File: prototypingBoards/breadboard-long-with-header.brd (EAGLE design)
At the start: 99.1 x 56.5 mm, 85 parts

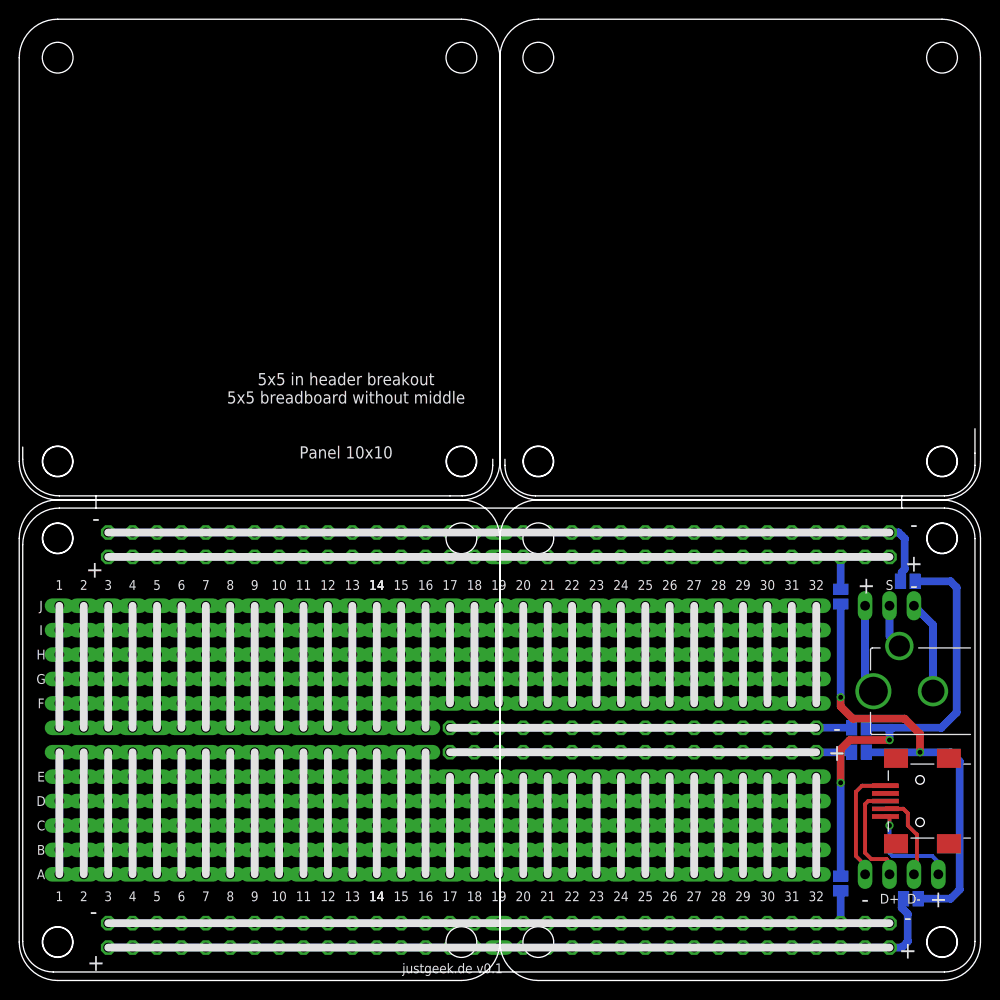
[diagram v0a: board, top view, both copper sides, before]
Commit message: Cleaned up boards
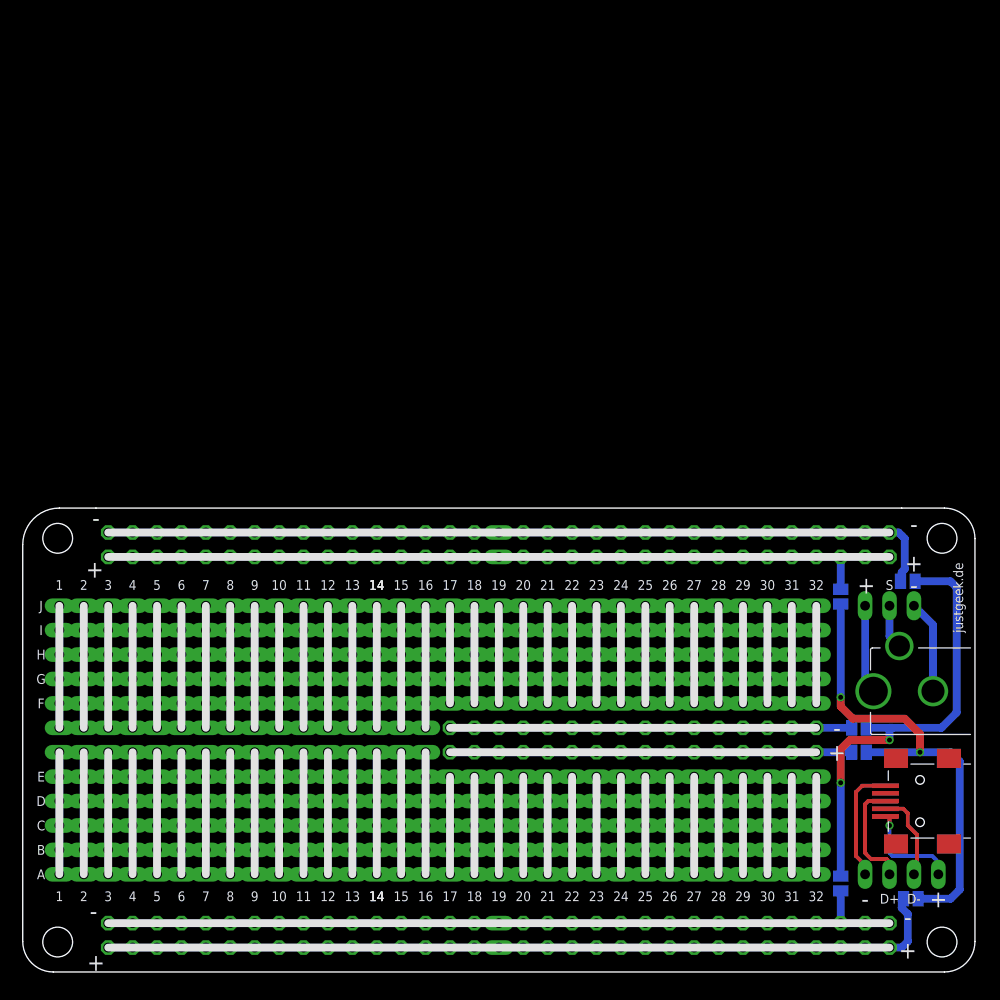
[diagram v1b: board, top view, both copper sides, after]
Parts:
- removed PCB1, PCB2, PCB3, PCB4: PCB_DP_SQUARE-5X5, dp_pcb:DP5050_V1
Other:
- board size 99.1 x 56.5 mm -> 99.1 x 48.3 mm
- board text added: "justgeek.de"
- board text removed: "5x5 in header breakout 5x5 breadboard without middle Panel 10x10"
- board text removed: "justgeek.de v0.1"
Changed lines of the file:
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@@
 <?xml version="1.0" encoding="utf-8"?>
 <!DOCTYPE eagle SYSTEM "eagle.dtd">
-<eagle version="6.5.0">
+<eagle version="7.1.0">
 <drawing>
 <settings>
@@
 <setting verticaltext="up"/>
 </settings>
-<grid distance="25" unitdist="mil" unit="mil" style="lines" multiple="1" display="yes" altdistance="5" altunitdist="mil" altunit="mil"/>
+<grid distance="1" unitdist="mm" unit="mm" style="lines" multiple="1" display="yes" altdistance="0.1" altunitdist="mm" altunit="mm"/>
 <layers>
 <layer number="1" name="Top" color="4" fill="1" visible="no" active="yes"/>
@@
 <layer number="19" name="Unrouted" color="6" fill="1" visible="no" active="yes"/>
 <layer number="20" name="Dimension" color="15" fill="1" visible="yes" active="yes"/>
-<layer number="21" name="tPlace" color="7" fill="1" visible="yes" active="yes"/>
+<layer number="21" name="tPlace" color="7" fill="1" visible="no" active="yes"/>
 <layer number="22" name="bPlace" color="7" fill="1" visible="yes" active="yes"/>
-<layer number="23" name="tOrigins" color="15" fill="1" visible="yes" active="yes"/>
+<layer number="23" name="tOrigins" color="15" fill="1" visible="no" active="yes"/>
 <layer number="24" name="bOrigins" color="15" fill="1" visible="no" active="yes"/>
-<layer number="25" name="tNames" color="7" fill="1" visible="yes" active="yes"/>
-<layer number="26" name="bNames" color="7" fill="1" visible="no" active="yes"/>
+<layer number="25" name="tNames" color="7" fill="1" visible="no" active="yes"/>
+<layer number="26" name="bNames" color="7" fill="1" visible="yes" active="yes"/>
 <layer number="27" name="tValues" color="7" fill="1" visible="no" active="yes"/>
-<layer number="28" name="bValues" color="7" fill="1" visible="no" active="yes"/>
-<layer number="29" name="tStop" color="7" fill="3" visible="yes" active="yes"/>
-<layer number="30" name="bStop" color="7" fill="6" visible="no" active="yes"/>
+<layer number="28" name="bValues" color="7" fill="1" visible="yes" active="yes"/>
+<layer number="29" name="tStop" color="7" fill="3" visible="no" active="yes"/>
+<layer number="30" name="bStop" color="7" fill="6" visible="yes" active="yes"/>
 <layer number="31" name="tCream" color="7" fill="4" visible="no" active="yes"/>
 <layer number="32" name="bCream" color="7" fill="5" visible="no" active="yes"/>
@@
 <layer number="43" name="vRestrict" color="2" fill="10" visible="no" active="yes"/>
 <layer number="44" name="Drills" color="7" fill="1" visible="no" active="yes"/>
-<layer number="45" name="Holes" color="7" fill="1" visible="yes" active="yes"/>
+<layer number="45" name="Holes" color="7" fill="1" visible="no" active="yes"/>
 <layer number="46" name="Milling" color="3" fill="1" visible="no" active="yes"/>
 <layer number="47" name="Measures" color="7" fill="1" visible="no" active="yes"/>
@@
 <layer number="109" name="ref-old" color="11" fill="1" visible="no" active="yes"/>
 <layer number="116" name="Patch_BOT" color="9" fill="4" visible="no" active="yes"/>
-<layer number="121" name="_tsilk" color="7" fill="1" visible="yes" active="yes"/>
-<layer number="122" name="_bsilk" color="7" fill="1" visible="no" active="yes"/>
+<layer number="121" name="_tsilk" color="7" fill="1" visible="no" active="yes"/>
+<layer number="122" name="_bsilk" color="7" fill="1" visible="yes" active="yes"/>
 <layer number="125" name="_tNames" color="7" fill="1" visible="no" active="yes"/>
 <layer number="131" name="prix" color="7" fill="1" visible="no" active="yes"/>
@@
 <text x="84.074" y="26.035" size="1.778" layer="21" font="vector" ratio="12" rot="R180" align="center">-</text>
 <text x="84.074" y="23.495" size="1.778" layer="21" font="vector" ratio="12" align="center">+</text>
-<text x="44.069" y="1.016" size="1.016" layer="21" font="vector" ratio="12" align="center">justgeek.de v0.1</text>
+<text x="96.684" y="39.569" size="1.016" layer="21" font="vector" ratio="12" rot="R90" align="center">justgeek.de</text>
 <text x="38.735" y="40.894" size="1.016" layer="21" font="vector" ratio="12" align="center">15</text>
 <text x="36.195" y="40.894" size="1.016" layer="21" font="vector" ratio="12" align="center">14</text>
@@
 <text x="79.375" y="8.509" size="1.016" layer="22" font="vector" ratio="12" rot="MR0" align="center">31</text>
 <text x="81.915" y="8.509" size="1.016" layer="22" font="vector" ratio="12" rot="MR0" align="center">32</text>
-<text x="33" y="58.5" size="1.27" layer="21" font="vector" ratio="12" align="center">5x5 in header breakout
-5x5 breadboard without middle
-Panel 10x10</text>
 <hole x="95" y="45.75" drill="3.1"/>
 <hole x="95" y="3.75" drill="3.1"/>
 <hole x="3" y="3.75" drill="3.1"/>
 <hole x="3" y="45.75" drill="3.1"/>
-<wire x1="3.175" y1="50.165" x2="6.985" y2="50.165" width="0" layer="20"/>
-<wire x1="6.985" y1="50.165" x2="6.985" y2="48.895" width="0" layer="20"/>
-<wire x1="90.805" y1="48.895" x2="90.805" y2="50.165" width="0" layer="20"/>
-<wire x1="90.805" y1="50.165" x2="95.25" y2="50.165" width="0" layer="20"/>
-<wire x1="48.26" y1="53.975" x2="48.26" y2="53.34" width="0" layer="20"/>
-<wire x1="48.26" y1="53.34" x2="45.085" y2="50.165" width="0" layer="20" curve="-90"/>
-<wire x1="45.085" y1="50.165" x2="43.815" y2="50.165" width="0" layer="20"/>
-<wire x1="49.53" y1="53.975" x2="49.53" y2="53.34" width="0" layer="20"/>
-<wire x1="49.53" y1="53.34" x2="52.705" y2="50.165" width="0" layer="20" curve="90"/>
-<wire x1="52.705" y1="50.165" x2="90.805" y2="50.165" width="0" layer="20"/>
-<wire x1="43.815" y1="50.165" x2="6.985" y2="50.165" width="0" layer="20"/>
-<hole x="3" y="53.75" drill="3.1"/>
-<hole x="45" y="53.75" drill="3.1"/>
-<hole x="53" y="53.75" drill="3.1"/>
-<hole x="95" y="53.75" drill="3.1"/>
-<wire x1="95.25" y1="50.165" x2="98.425" y2="53.34" width="0" layer="20" curve="90"/>
-<wire x1="98.425" y1="53.34" x2="98.425" y2="54.61" width="0" layer="20"/>
-<wire x1="98.425" y1="54.61" x2="98.425" y2="57.15" width="0" layer="20"/>
-<wire x1="3.175" y1="50.165" x2="-0.635" y2="53.975" width="0" layer="20" curve="-90"/>
-<wire x1="-0.635" y1="53.975" x2="-0.635" y2="55.245" width="0" layer="20"/>
 </plain>
 <attributes>
@@
 <pass name="Default">
 <param name="RoutingGrid" value="25mil"/>
+<param name="AutoGrid" value="1"/>
+<param name="Efforts" value="0"/>
+<param name="TopRouterVariant" value="1"/>
 <param name="tpViaShape" value="round"/>
 <param name="PrefDir.1" value="|"/>
@@
 <attribute name="VALUE" x="46.355" y="4.445" size="0.8" layer="27" font="vector" rot="R270" align="center"/>
 </element>
-<element name="PCB1" library="dp_pcb" package="DP5050_V1" value="PCB_DP_SQUARE-5X5" x="-1" y="-0.25"/>
-<element name="PCB2" library="dp_pcb" package="DP5050_V1" value="PCB_DP_SQUARE-5X5" x="49" y="-0.25"/>
-<element name="PCB3" library="dp_pcb" package="DP5050_V1" value="PCB_DP_SQUARE-5X5" x="-1" y="49.75"/>
-<element name="PCB4" library="dp_pcb" package="DP5050_V1" value="PCB_DP_SQUARE-5X5" x="49" y="49.75"/>
 </elements>
 <signals>
@@
 </board>
 </drawing>
-<compatibility>
-<note version="6.3" minversion="6.2.2" severity="warning">
-Since Version 6.2.2 text objects can contain more than one line,
-which will not be processed correctly with this version.
-</note>
-</compatibility>
 </eagle>
